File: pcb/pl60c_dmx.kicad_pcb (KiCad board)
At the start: 2 copper layers, 80 x 54 mm, 39 parts, among them J1 USB-C 16P, J2 XLR-5 female (DMX OUT), J3 DMX pigtail, J4 EXPANSION, J5 UART0, Q1 S8050, SW1 RESET, SW2 BOOT, SW3 USER, U1 ESP32-S3-WROOM-1-N16R8, U2 AMS1117-3.3, U3 SP3485EN, U4 USBLC6-2SC6

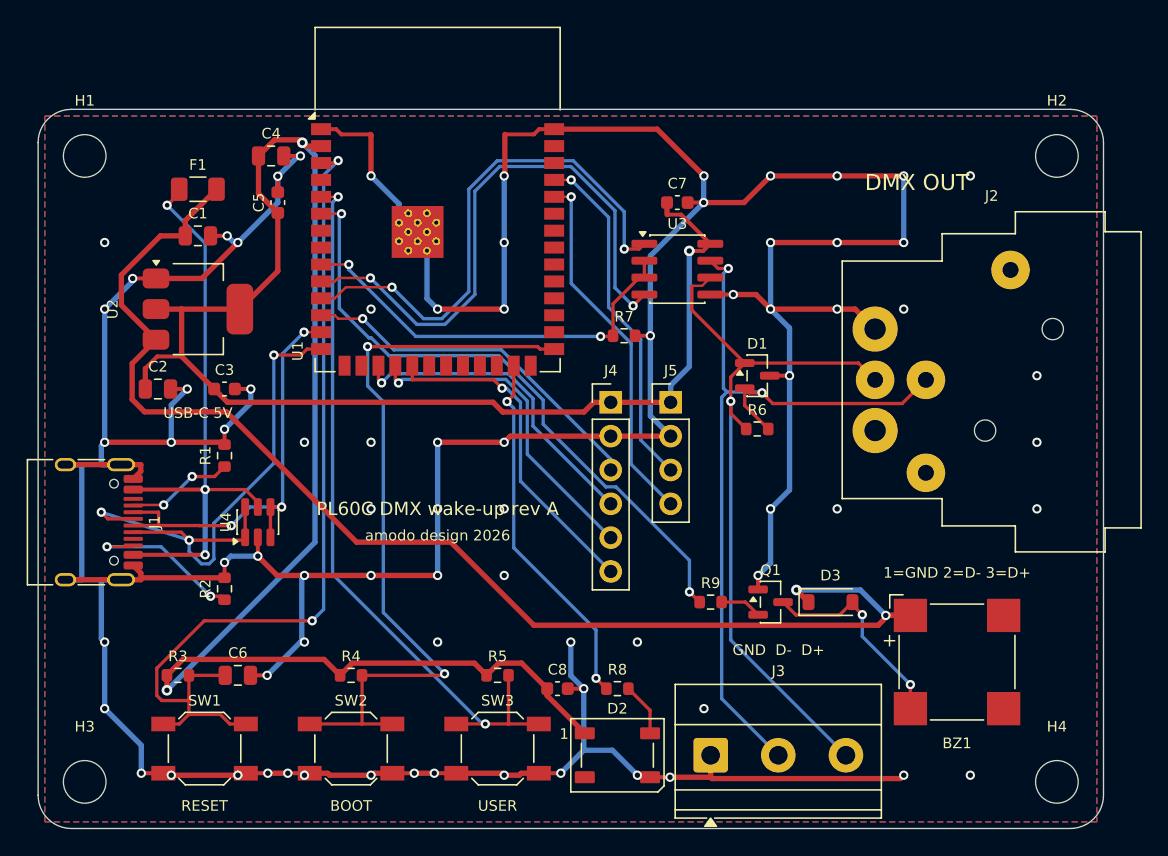
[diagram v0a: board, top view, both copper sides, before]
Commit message: auto: 2026-09-02 14:26:12
Co-Authored-By: Claude Fable 5.1 <noreply@anthropic.com>
Claude-Session: https://claude.ai/code/session_01WsrVZb94LwbHVAmBvsSTfn
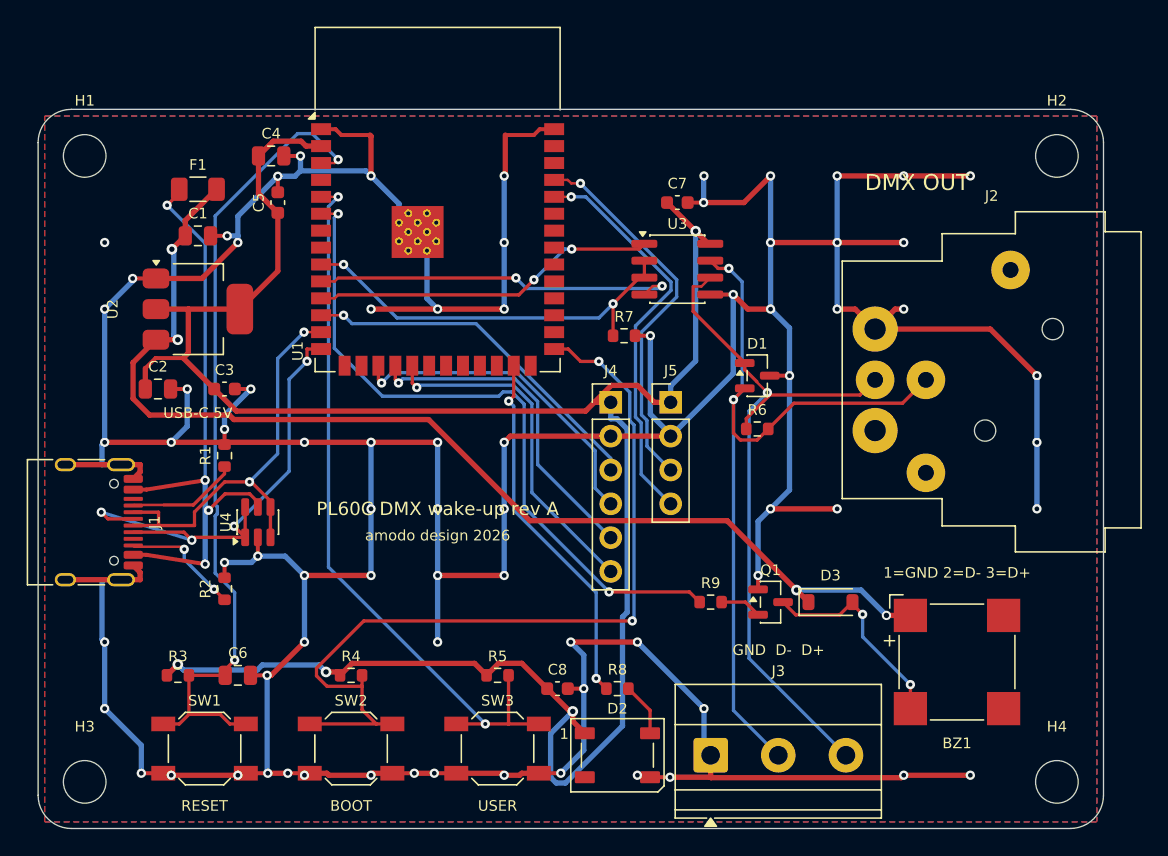
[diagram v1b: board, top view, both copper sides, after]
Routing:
- net GND: track 395.7 -> 472.7 mm
- net DMX_TX: track 43.4 -> 27.7 mm
- net DMX_RX: track 39.6 -> 26.0 mm
- net +5V: track 98.1 -> 86.0 mm, vias 2 -> 4
- net +3V3: track 174.0 -> 166.7 mm, vias 3 -> 4
- net IO0_BOOT: track 57.1 -> 64.2 mm
- net USB_D+: track 44.7 -> 38.5 mm, vias 3 -> 4
- net EN: track 66.9 -> 62.0 mm
- net BUZZER: track 47.3 -> 51.6 mm
- net CC2: track 12.5 -> 9.05 mm
- net VBUS: track 44.5 -> 47.8 mm, vias 3 -> 4
- net RXD0: track 27.4 -> 30.3 mm
- net TXD0: track 26.2 -> 28.6 mm
- net DMX_B: track 61.6 -> 60.5 mm
- net DMX_A: track 55.4 -> 54.6 mm
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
